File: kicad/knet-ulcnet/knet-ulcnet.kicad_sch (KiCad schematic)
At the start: 11 parts, among them J1 Conn_01x04, U11 SIO0-DIP-40, X1 SN65LBC176P, X11 SIO0-DIP-40, X2 SN65LBC176P, X3 74LS123

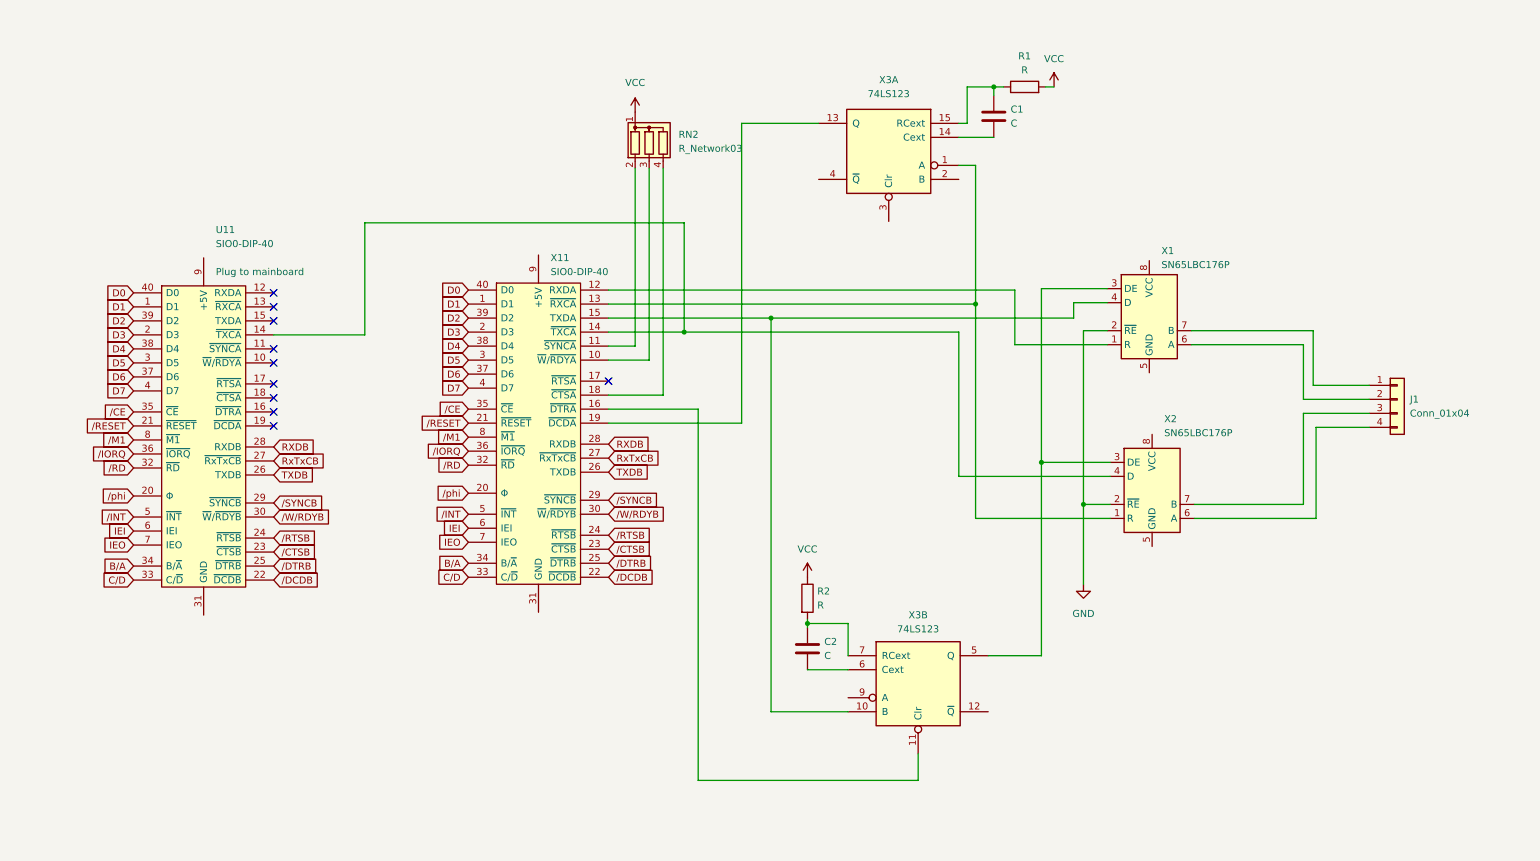
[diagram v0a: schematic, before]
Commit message: working KayNetSerial, updated schematic
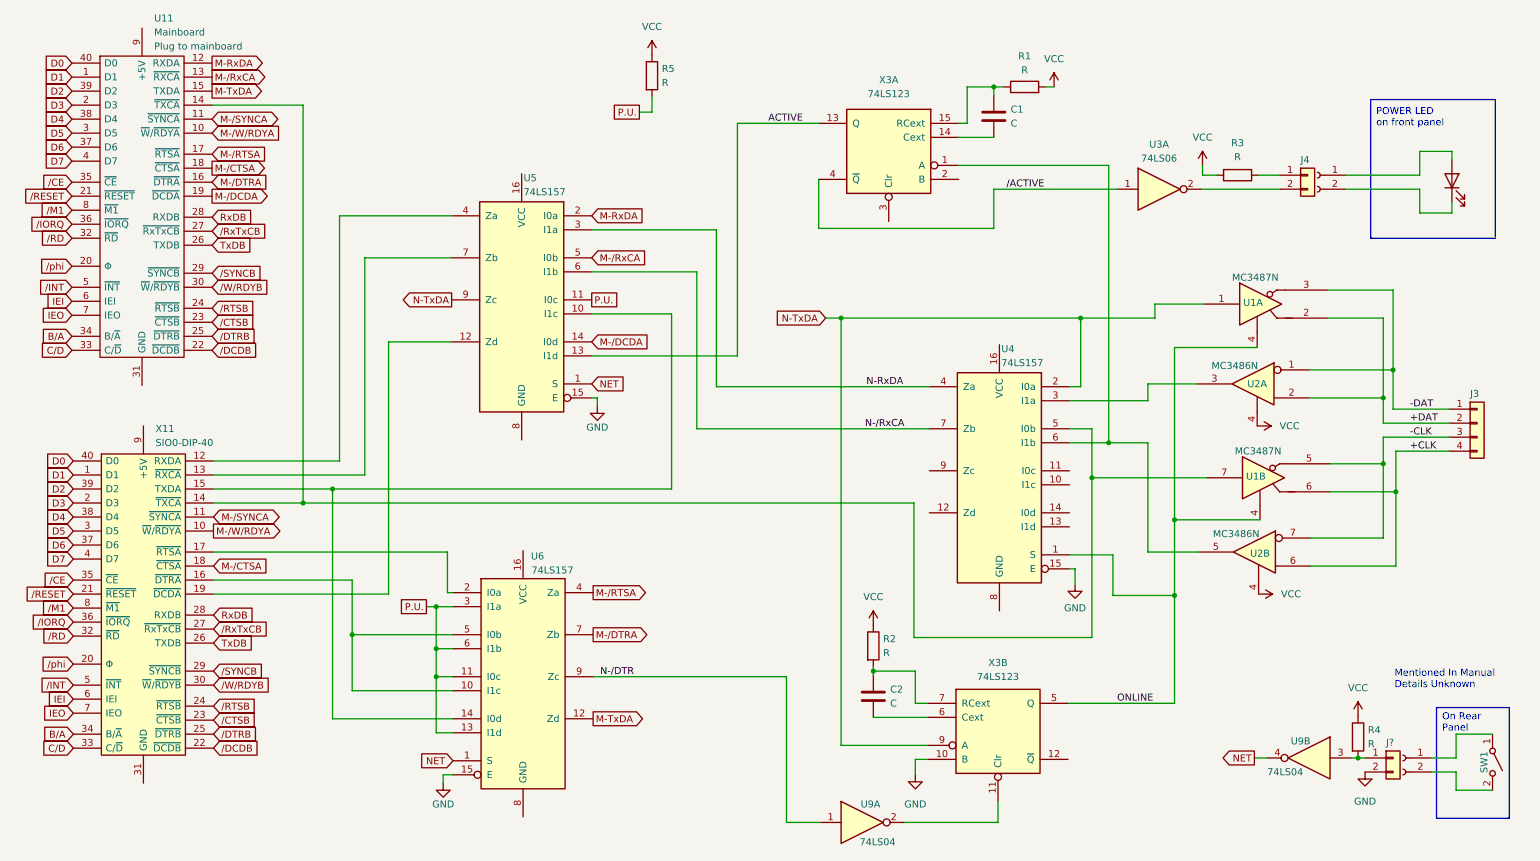
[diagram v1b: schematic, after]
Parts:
- removed RN2: R_Network03, Resistor_THT:R_Array_SIP4, symbol Device:R_Network03
- removed X1, X2: SN65LBC176P, Package_DIP:DIP-8_W7.62mm, symbol Interface_UART:SN65LBC176P
- added D1: LED, symbol Device:LED
- added J1, J5: Conn_01x02_Socket, symbol Connector:Conn_01x02_Socket
- added J4, J?: Conn_01x02, symbol Connector_Generic:Conn_01x02
- added R3, R4, R5: R, symbol Device:R
- added SW1: SW_SPST, symbol Switch:SW_SPST
- added U1: MC3487N, Package_DIP:DIP-16_W7.62mm, symbol Interface_LineDriver:MC3487N
- added U2: MC3486N, Package_DIP:DIP-14_W7.62mm, symbol Interface_LineDriver:MC3486N
- added U3: 74LS06, symbol 74xx:74LS06
- added U4, U5, U6: 74LS157, symbol 74xx:74LS157
- added U9: 74LS04, symbol 74xx:74LS04
- U11: value SIO0-DIP-40 -> Mainboard
- renumbered J1 to J3
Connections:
- net GND: now also X3.10 (B), J?.2 (Pin_2), U4.15 (E), U5.15 (E), U6.15 (E)
- net VCC: now also R3.2, R4.1, R5.1, U2.4 (ENABLE), U2.4 (ENABLE)
- net at X3.1 (A): now also U2.5 (OUT), U4.6 (I1b); no longer X11.13 (~{RXCA})
- net ONLINE: now reaches X3.5 (Q)
- net ONLINE: now also U1.4 (ENABLE), U1.4 (ENABLE), U4.1 (S)
- net at U11.14 (~{TXCA}), X11.14 (~{TXCA}): now also U1.7 (INPUT), U4.5 (I0b)
- net +CLK: now reaches J3.4 (Pin_4)
- net +CLK: now also U1.6 (OUT+), U2.6 (E+)
- net -CLK: now reaches J3.3 (Pin_3)
- net -CLK: now also U1.5 (OUT-), U2.7 (E-)
- net M-/W/RDYA: now reaches X11.10 (~{W}/~{RDYA})
- net M-/W/RDYA: now also U11.10 (~{W}/~{RDYA})
- net M-/SYNCA: now reaches X11.11 (~{SYNCA})
- net M-/SYNCA: now also U11.11 (~{SYNCA})
- net at X11.12 (RXDA): now also U5.4 (Za)
- net at X11.15 (TXDA): now also U5.10 (I1c), U6.14 (I0d); no longer X3.10 (B)
- net at X11.16 (~{DTRA}): now also U6.10 (I1c), U6.5 (I0b); no longer X3.11 (Clr)
- net at X11.17 (~{RTSA}): now also U6.2 (I0a)
- net M-/CTSA: now reaches X11.18 (~{CTSA})
- net M-/CTSA: now also U11.18 (~{CTSA})
- net at X11.19 (~{DCDA}): now also U5.12 (Zd); no longer X3.13 (Q)
- net N-TxDA: now reaches X3.9 (A)
- net N-TxDA: now also U1.1 (INPUT), U4.2 (I0a), U5.9 (Zc)
- net /ACTIVE: now reaches X3.4 (~{Q})
- net /ACTIVE: now also U3.1
- net -DAT: now reaches J3.1 (Pin_1)
- net -DAT: now also U1.3 (OUT-), U2.1 (E-)
- net +DAT: now reaches J3.2 (Pin_2)
- net +DAT: now also U1.2 (OUT+), U2.2 (E+)
- net M-RxDA: now reaches U11.12 (RXDA)
- net M-RxDA: now also U5.2 (I0a)
- net M-/RxCA: now reaches U11.13 (~{RXCA})
- net M-/RxCA: now also U5.5 (I0b)
- net M-TxDA: now reaches U11.15 (TXDA)
- net M-TxDA: now also U6.12 (Zd)
- net M-/DTRA: now reaches U11.16 (~{DTRA})
- net M-/DTRA: now also U6.7 (Zb)
- net M-/RTSA: now reaches U11.17 (~{RTSA})
- net M-/RTSA: now also U6.4 (Za)
- net M-/DCDA: now reaches U11.19 (~{DCDA})
- net M-/DCDA: now also U5.14 (I0d)
- net RXDB renamed RxDB
- net RxTxCB renamed /RxTxCB
- net TXDB renamed TxDB
- new net: U2.3 (OUT), U4.3 (I1a)
- new net: U5.7 (Zb), X11.13 (~{RXCA})
- new net: U9.2, X3.11 (Clr)
- new net: D1.1 (K), J1.2 (Pin_2)
- new net: D1.2 (A), J1.1 (Pin_1)
- new net: J5.1 (Pin_1), SW1.1 (A)
- new net: J5.2 (Pin_2), SW1.2 (B)
- new net: J?.1 (Pin_1), R4.2, U9.3
- new net: J4.1 (Pin_1), R3.1
- new net: J4.2 (Pin_2), U3.2
- new net ACTIVE: U5.13 (I1d), X3.13 (Q)
- new net N-RxDA: U4.4 (Za), U5.3 (I1a)
- new net N-/DTR: U6.9 (Zc), U9.1
- new net N-/RxCA: U4.7 (Zb), U5.6 (I1b)
- new net NET: U5.1 (S), U6.1 (S), U9.4
- new net P.U.: R5.2, U5.11 (I0c), U6.11 (I0c), U6.13 (I1d), U6.3 (I1a), U6.6 (I1b)
- no-connect marks 10 -> 0
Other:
- note added: "Mentioned In Manual Details Unknown"
- note added: "On Rear Panel"
- note added: "POWER LED on front panel"
- moved on the sheet: C2, J3, R2, X11, X3B
